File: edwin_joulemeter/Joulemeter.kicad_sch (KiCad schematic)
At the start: 56 parts, among them J1 XT60-M, J2 22035035, J3 22035035, J4 XT60-M, U1 INA240A1PWR, U3 MCP6286T-E/OT, U4 PADS131M04QPWRQ1

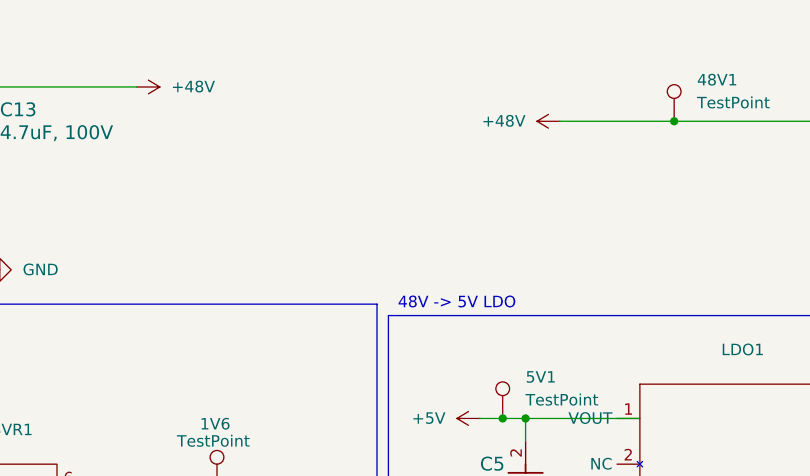
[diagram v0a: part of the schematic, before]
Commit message: third update 1/25/25
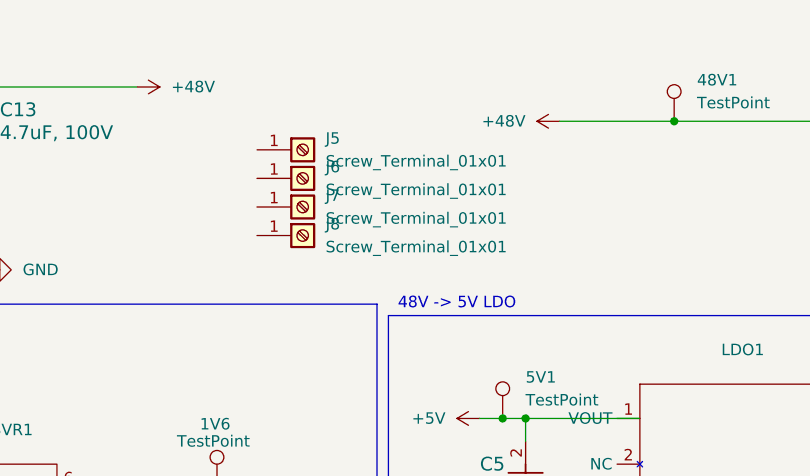
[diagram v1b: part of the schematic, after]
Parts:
- added J5, J6, J7, J8: Screw_Terminal_01x01, TerminalBlock_MetzConnect:TerminalBlock_MetzConnect_360271_1x01_Horizontal_ScrewM3.0_Boxed, symbol Connector:Screw_Terminal_01x01

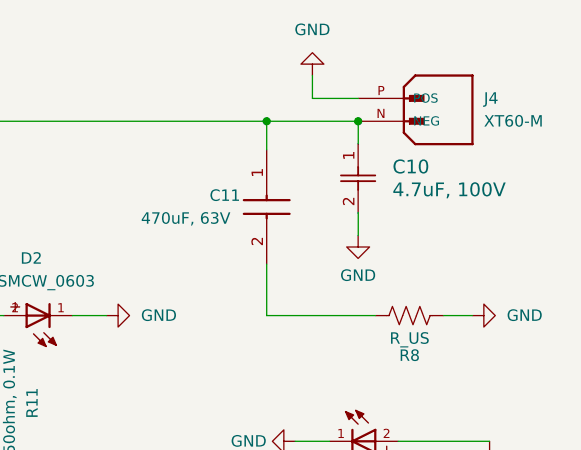
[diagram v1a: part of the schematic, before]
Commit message: small error lol
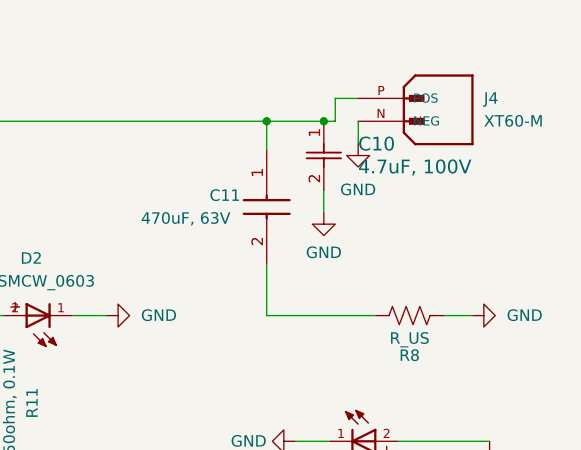
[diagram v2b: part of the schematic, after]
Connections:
- net GND: now also J4.N (NEG); no longer J4.P (POS)
- net SHUNT_OUT: now also J4.P (POS); no longer J4.N (NEG)
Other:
- moved on the sheet: C10
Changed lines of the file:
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@@
 	)
 	(junction
-		(at 262.89 25.4)
-		(diameter 0)
-		(color 0 0 0 0)
-	)
-	(junction
 		(at 30.48 162.56)
 		(diameter 0)
@@
 	)
 	(junction
+		(at 259.08 25.4)
+		(diameter 0)
+		(color 0 0 0 0)
+	)
+	(junction
 		(at 220.345 67.31)
 		(diameter 0)
@@
 	)
 	(junction
-		(at 252.73 25.4)
+		(at 35.56 162.56)
 		(diameter 0)
 		(color 0 0 0 0)
 	)
 	(junction
-		(at 35.56 162.56)
+		(at 113.03 156.21)
 		(diameter 0)
 		(color 0 0 0 0)
 	)
 	(junction
-		(at 113.03 156.21)
+		(at 252.73 25.4)
 		(diameter 0)
 		(color 0 0 0 0)
@@
 	(wire
 		(pts
-			(xy 262.89 22.86) (xy 257.81 22.86)
+			(xy 24.13 66.04) (xy 24.13 66.675)
 		)
 		(stroke
@@
 	(wire
 		(pts
-			(xy 24.13 66.04) (xy 24.13 66.675)
+			(xy 100.33 116.84) (xy 100.33 123.19)
 		)
 		(stroke
@@
 	(wire
 		(pts
-			(xy 100.33 116.84) (xy 100.33 123.19)
+			(xy 259.08 25.4) (xy 260.35 25.4)
 		)
 		(stroke
@@
 	(wire
 		(pts
+			(xy 252.73 25.4) (xy 259.08 25.4)
+		)
+		(stroke
+			(width 0)
+			(type default)
+		)
+	)
+	(wire
+		(pts
 			(xy 142.24 106.68) (xy 142.24 107.95)
 		)
@@
 	(wire
 		(pts
+			(xy 260.35 22.86) (xy 260.35 25.4)
+		)
+		(stroke
+			(width 0)
+			(type default)
+		)
+	)
+	(wire
+		(pts
 			(xy 275.59 139.7) (xy 275.59 144.78)
 		)
@@
 	(wire
 		(pts
-			(xy 262.89 35.56) (xy 262.89 38.1)
+			(xy 259.08 33.02) (xy 259.08 35.56)
 		)
 		(stroke
@@
 	(wire
 		(pts
-			(xy 252.73 25.4) (xy 262.89 25.4)
-		)
-		(stroke
-			(width 0)
-			(type default)
-		)
-	)
-	(wire
-		(pts
 			(xy 40.64 66.04) (xy 45.085 66.04)
 		)
@@
 	(wire
 		(pts
+			(xy 260.35 22.86) (xy 262.89 22.86)
+		)
+		(stroke
+			(width 0)
+			(type default)
+		)
+	)
+	(wire
+		(pts
 			(xy 77.47 127) (xy 77.47 128.27)
 		)
@@
 	(wire
 		(pts
-			(xy 257.81 22.86) (xy 257.81 20.32)
+			(xy 262.89 25.4) (xy 262.89 27.94)
 		)
 		(stroke
@@
 	(wire
 		(pts
-			(xy 262.89 25.4) (xy 262.89 27.94)
-		)
-		(stroke
-			(width 0)
-			(type default)
-		)
-	)
-	(wire
-		(pts
 			(xy 200.66 25.4) (xy 200.66 36.83)
 		)
@@
 	(symbol
 		(lib_id "power:GND")
-		(at 262.89 38.1 0)
+		(at 259.08 35.56 0)
 		(unit 1)
 		(exclude_from_sim no)
@@
 		(dnp no)
 		(property "Reference" "#PWR036"
-			(at 262.89 44.45 0)
+			(at 259.08 41.91 0)
 			(effects
 				(font
@@
 		)
 		(property "Value" "GND"
-			(at 262.89 42.545 0)
+			(at 259.08 40.005 0)
 			(effects
 				(font
@@
 		)
 		(property "Footprint" ""
-			(at 262.89 38.1 0)
+			(at 259.08 35.56 0)
 			(effects
 				(font
@@
 		)
 		(property "Datasheet" ""
-			(at 262.89 38.1 0)
+			(at 259.08 35.56 0)
 			(effects
 				(font
@@
 		)
 		(property "Description" "Power symbol creates a global label with name \"GND\" , ground"
-			(at 262.89 38.1 0)
+			(at 259.08 35.56 0)
 			(effects
 				(font
@@
 	(symbol
 		(lib_id "power:GND")
-		(at 257.81 20.32 180)
+		(at 262.89 27.94 0)
 		(unit 1)
 		(exclude_from_sim no)
@@
 		(fields_autoplaced yes)
 		(property "Reference" "#PWR032"
-			(at 257.81 13.97 0)
+			(at 262.89 34.29 0)
 			(effects
 				(font
@@
 		)
 		(property "Value" "GND"
-			(at 257.81 15.24 0)
+			(at 262.89 33.02 0)
 			(effects
 				(font
@@
 		)
 		(property "Footprint" ""
-			(at 257.81 20.32 0)
+			(at 262.89 27.94 0)
 			(effects
 				(font
@@
 		)
 		(property "Datasheet" ""
-			(at 257.81 20.32 0)
+			(at 262.89 27.94 0)
 			(effects
 				(font
@@
 		)
 		(property "Description" "Power symbol creates a global label with name \"GND\" , ground"
-			(at 257.81 20.32 0)
+			(at 262.89 27.94 0)
 			(effects
 				(font
@@
 	(symbol
 		(lib_id "SMV_Custom:C2220C475M1R2C7186")
-		(at 262.89 27.94 270)
+		(at 259.08 25.4 270)
 		(unit 1)
 		(exclude_from_sim no)
@@
 		(dnp no)
 		(property "Reference" "C10"
-			(at 266.7 30.4799 90)
+			(at 262.89 27.9399 90)
 			(effects
 				(font
@@
 		)
 		(property "Value" "4.7uF, 100V"
-			(at 266.7 33.0199 90)
+			(at 262.89 30.4799 90)
 			(effects
 				(font
@@
 		)
 		(property "Footprint" "CAP_C2220C_2S_KEM"
-			(at 262.89 27.94 0)
+			(at 259.08 25.4 0)
 			(effects
 				(font
@@
 		)
 		(property "Datasheet" "C2220C475M1R2C7186"
-			(at 262.89 27.94 0)
+			(at 259.08 25.4 0)
 			(effects
 				(font
@@
 		)
 		(property "Description" ""
-			(at 262.89 27.94 0)
+			(at 259.08 25.4 0)
 			(effects
 				(font
